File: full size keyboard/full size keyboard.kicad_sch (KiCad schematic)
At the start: 195 parts, among them SW1 SW_Nidec_CAS-120A1, U1 MIC29502WU, U10 CJ432, U11 CJ432, U12 CJ432, U13 CJ432, U14 CJ432, U15 CJ432, U16 CJ432, U17 CJ432, U18 CJ432, U19 CJ432, U2 CJ432, U20 CJ432, U21 CJ432, U22 CJ432, U23 CJ432, U24 CJ432, U25 CJ432, U26 CJ432, U27 CJ432, U28 CJ432, U29 CJ432, U3 CJ432, U30 CJ432, U31 CJ432, U32 CJ432, U33 CJ432, U34 CJ432, U35 CJ432, U36 CJ432, U37 CJ432, U38 CJ432, U39 CJ432, U4 CJ432, U40 CJ432, U41 CJ432, U42 CJ432, U43 CJ432, U44 CJ432, U45 CJ432, U46 CJ432, U47 CJ432, U48 CJ432, U49 CJ432, U5 CJ432, U50 CJ432, U51 CJ432, U52 CJ432, U53 CJ432, U54 CJ432, U55 CJ432, U56 CJ432, U57 CJ432, U58 CJ432, U59 CJ432, U6 CJ432, U60 CJ432, U61 CJ432, U62 CJ432, U7 CJ432, U8 CJ432, U9 CJ432

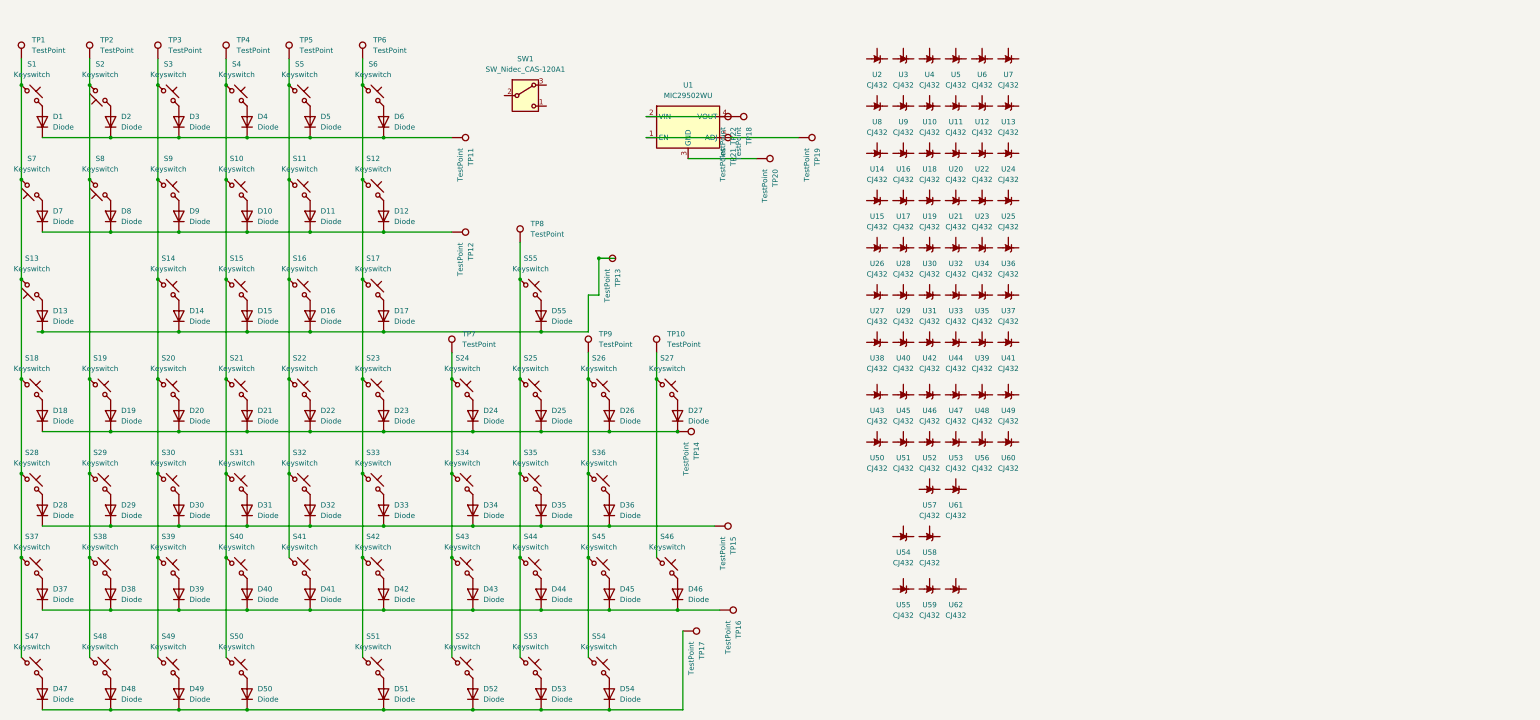
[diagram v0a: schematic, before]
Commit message: changes
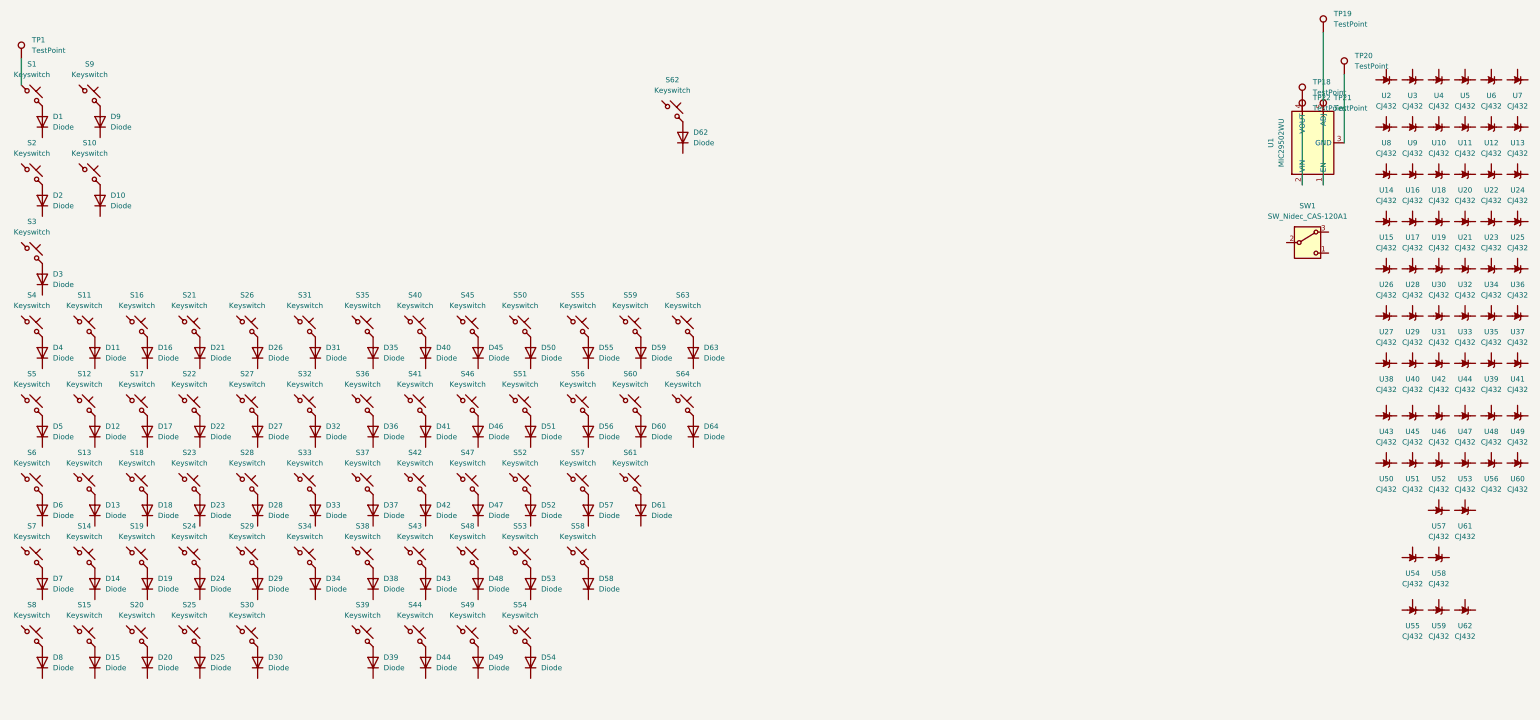
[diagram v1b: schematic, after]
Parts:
- removed TP10, TP11, TP12, TP13, TP14, TP15, TP16, TP17, TP2, TP3, TP4, TP5, TP6, TP7, TP8, TP9: TestPoint, TestPoint:TestPoint_Pad_D1.5mm, symbol Connector:TestPoint
- added D56, D57, D58, D59, D60, D61, D62, D63, D64: Diode, Diode_SMD:D_PowerDI-123, symbol ScottoKeebs:Placeholder_Diode
- added S56, S57, S58, S59, S60, S61, S62, S63, S64: Keyswitch, custom_footprints:8mm, symbol ScottoKeebs:Placeholder_Keyswitch
- S10, S11, S12, S14, S15, S16, S17, S18, S19, S20, S21, S22, S23, S24, S25, S26, S27, S28, S29, S3, S30, S31, S32, S33, S34, S35, S36, S37, S38, S39, S4, S40, S41, S42, S43, S44, S45, S47, S48, S49, S5, S52, S53, S54, S6, S9: footprint custom_footprints:3rd -> custom_footprints:8mm
- S13, S2, S7, S8: footprint custom_footprints:Triangle -> custom_footprints:8mm
- S50, S51: footprint custom_footprints:oblong 230 -> custom_footprints:8mm
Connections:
- net at S7.1: no longer D7.2 (A)
- net at S2.1: no longer D2.2 (A)
- net at D13.2 (A): now also S13.2; no longer S13.1
- net at S27.1: no longer S46.1
- net at D8.2 (A): now also S8.2; no longer S8.1
- new net: D57.2 (A), S57.2
- new net: D62.2 (A), S62.2
- new net: D2.2 (A), S2.2
- new net: D63.2 (A), S63.2
- new net: D61.2 (A), S61.2
- new net: D60.2 (A), S60.2
- new net: S1.1, TP1.1
- new net: D7.2 (A), S7.2
- new net: D58.2 (A), S58.2
- new net: D56.2 (A), S56.2
- new net: D64.2 (A), S64.2
- new net: D59.2 (A), S59.2
- now unconnected: D1.1 (K), D10.1 (K), D11.1 (K), D12.1 (K), D13.1 (K), D14.1 (K), D15.1 (K), D16.1 (K), D17.1 (K), D18.1 (K), D19.1 (K), D2.1 (K), D20.1 (K), D21.1 (K), D22.1 (K), D23.1 (K), D24.1 (K), D25.1 (K), D26.1 (K), D27.1 (K), D28.1 (K), D29.1 (K), D3.1 (K), D30.1 (K), D31.1 (K), D32.1 (K), D33.1 (K), D34.1 (K), D35.1 (K), D36.1 (K), D37.1 (K), D38.1 (K), D39.1 (K), D4.1 (K), D40.1 (K), D41.1 (K), D42.1 (K), D43.1 (K), D44.1 (K), D45.1 (K), D46.1 (K), D47.1 (K), D48.1 (K), D49.1 (K), D5.1 (K), D50.1 (K), D51.1 (K), D52.1 (K), D53.1 (K), D54.1 (K), D55.1 (K), D6.1 (K), D7.1 (K), D8.1 (K), D9.1 (K), S10.1, S11.1, S12.1, S14.1, S15.1, S16.1, S17.1, S18.1, S19.1, S20.1, S21.1, S22.1, S23.1, S24.1, S25.1, S26.1, S28.1, S29.1, S3.1, S30.1, S31.1, S32.1, S33.1, S34.1, S35.1, S36.1, S37.1, S38.1, S39.1, S4.1, S40.1, S41.1, S42.1, S43.1, S44.1, S45.1, S47.1, S48.1, S49.1, S5.1, S50.1, S51.1, S52.1, S53.1, S54.1, S55.1, S6.1, S9.1
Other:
- moved on the sheet: SW1, TP18, TP19, TP20, TP21, TP22, U1, U10, U11, U12, U13, U14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
